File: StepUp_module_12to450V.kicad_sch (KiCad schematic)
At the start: 0 parts

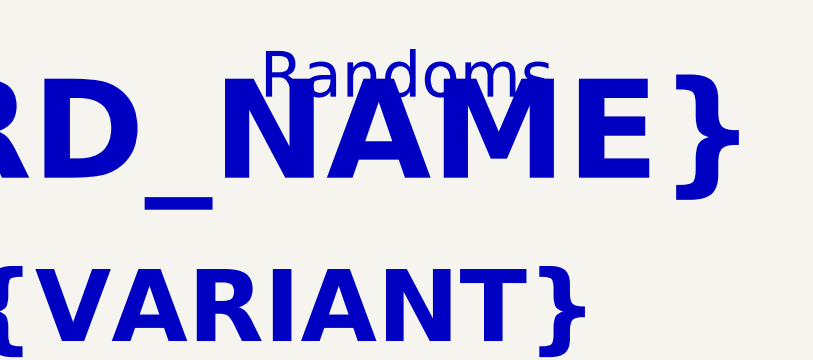
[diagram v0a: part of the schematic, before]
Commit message: DBG18
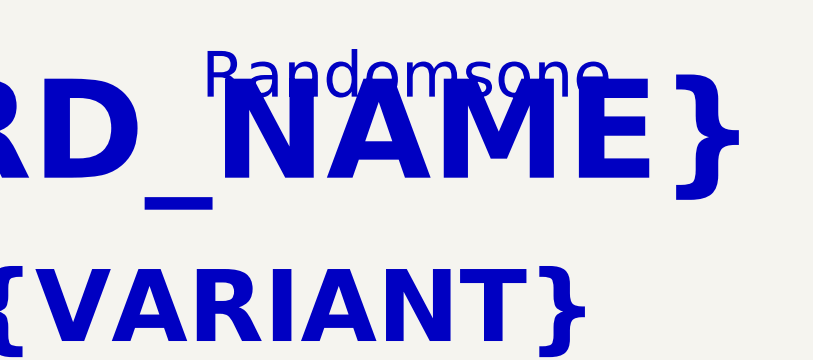
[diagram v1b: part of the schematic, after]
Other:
- note added: "Randomsone"
- note removed: "Randoms"
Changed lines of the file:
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@@
 		)
 	)
-	(text "Randoms"
+	(text "Randomsone"
 		(exclude_from_sim no)
 		(at 135.89 27.94 0)

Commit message: Preping release 1.0.0
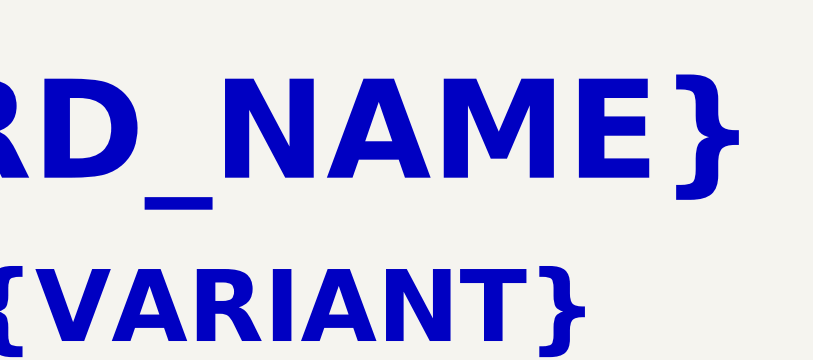
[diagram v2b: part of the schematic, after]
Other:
- note removed: "Randomsone"
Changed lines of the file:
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@@
-		)
-	)
-	(text "Randomsone"
-		(exclude_from_sim no)
-		(at 135.89 27.94 0)
-		(effects
-			(font
-				(size 5.08 5.08)
-			)
 		)
 	)
